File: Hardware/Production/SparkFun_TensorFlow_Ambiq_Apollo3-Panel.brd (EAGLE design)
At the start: 175.6 x 134.7 mm, 906 parts, among them J12 CORTEX_DEBUG, J14 CAMERA-OV7670, J18 CORTEX_DEBUG, J20 CAMERA-OV7670, J24 CORTEX_DEBUG, J26 CAMERA-OV7670, J30 CORTEX_DEBUG, J32 CAMERA-OV7670, J36 CORTEX_DEBUG, J38 CAMERA-OV7670, J42 CORTEX_DEBUG, J44 CAMERA-OV7670, J48 CORTEX_DEBUG, J5 CORTEX_DEBUG, J50 CAMERA-OV7670, J54 CORTEX_DEBUG, J6 CAMERA-OV7670, J8 CAMERA-OV7670, U1 LIS2DH12, U10 LIS2DH12, U11 1.8V, U12 ARTEMIS_MODULESMD, U13 LIS2DH12, U14 1.8V, U15 ARTEMIS_MODULESMD, U16 LIS2DH12, U17 1.8V, U18 ARTEMIS_MODULESMD, U19 LIS2DH12, U2 LIS2DH12, U20 1.8V, U21 ARTEMIS_MODULESMD, U22 LIS2DH12, U23 1.8V, U24 ARTEMIS_MODULESMD, U25 LIS2DH12, U26 1.8V, U27 ARTEMIS_MODULESMD, U3 1.8V, U4 1.8V, U5 ARTEMIS_MODULESMD, U6 ARTEMIS_MODULESMD, U7 LIS2DH12, U8 1.8V, U9 ARTEMIS_MODULESMD, Y1 32.768kHz, Y2 32.768kHz, Y3 32.768kHz, Y4 32.768kHz, Y5 32.768kHz, Y6 32.768kHz, Y7 32.768kHz, Y8 32.768kHz, Y9 32.768kHz

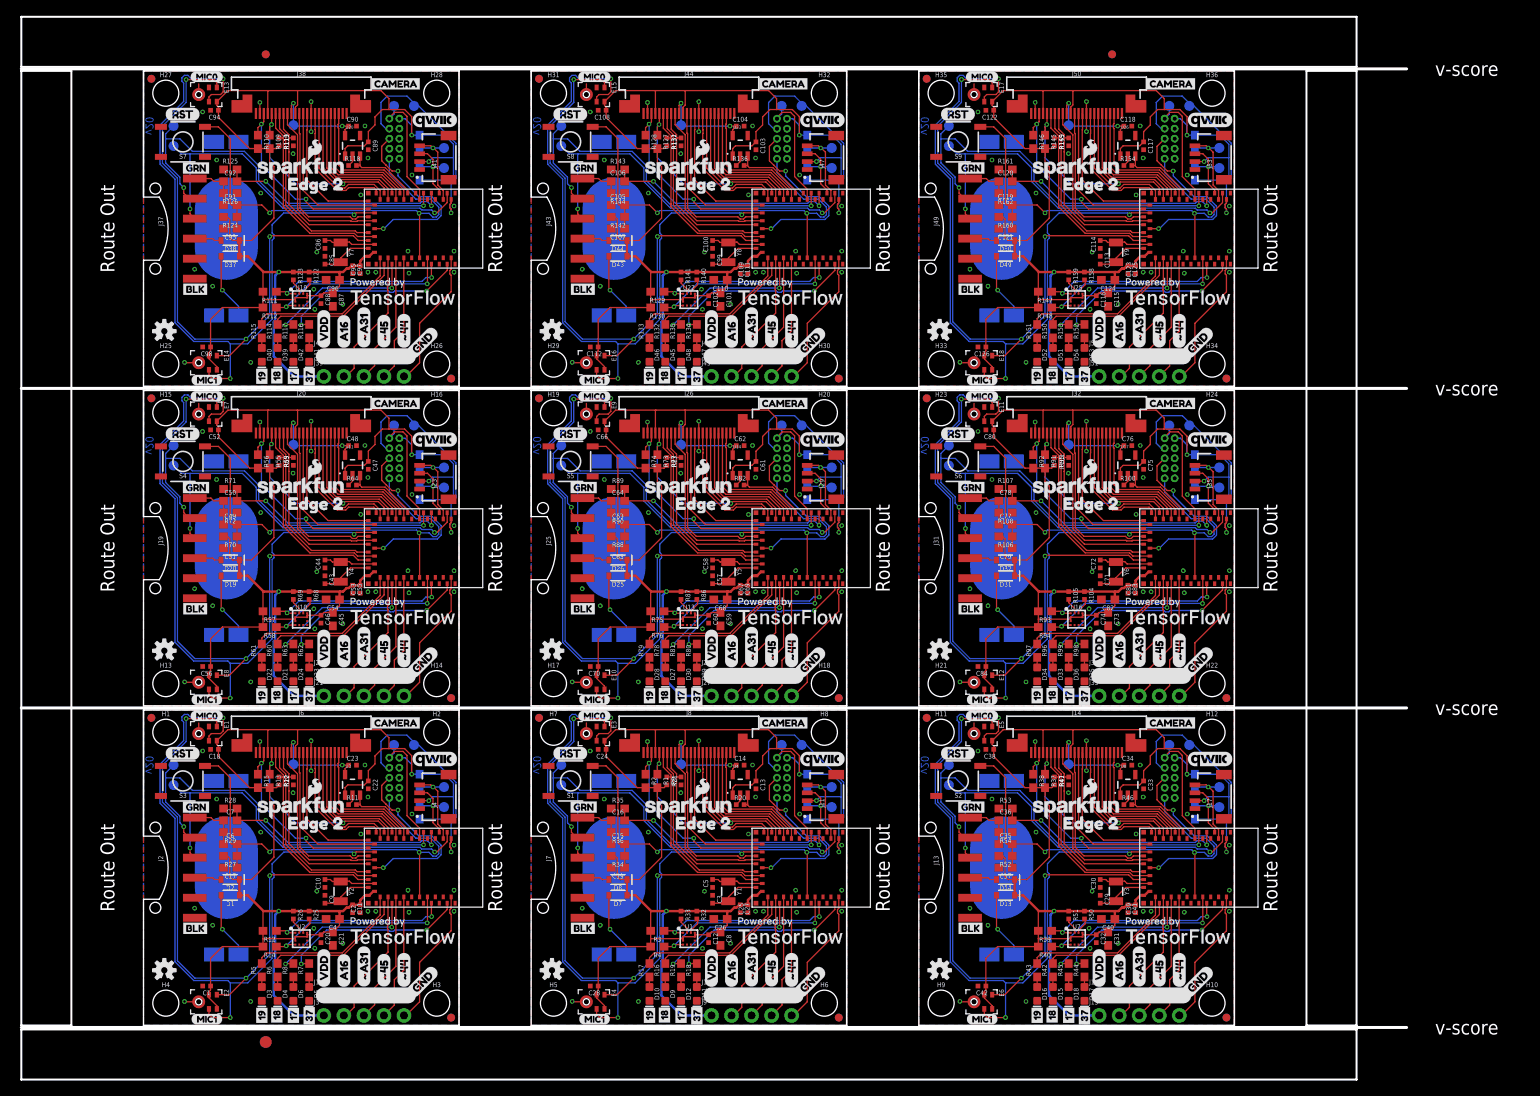
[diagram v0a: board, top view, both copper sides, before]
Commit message: Adding panel files for v2.1
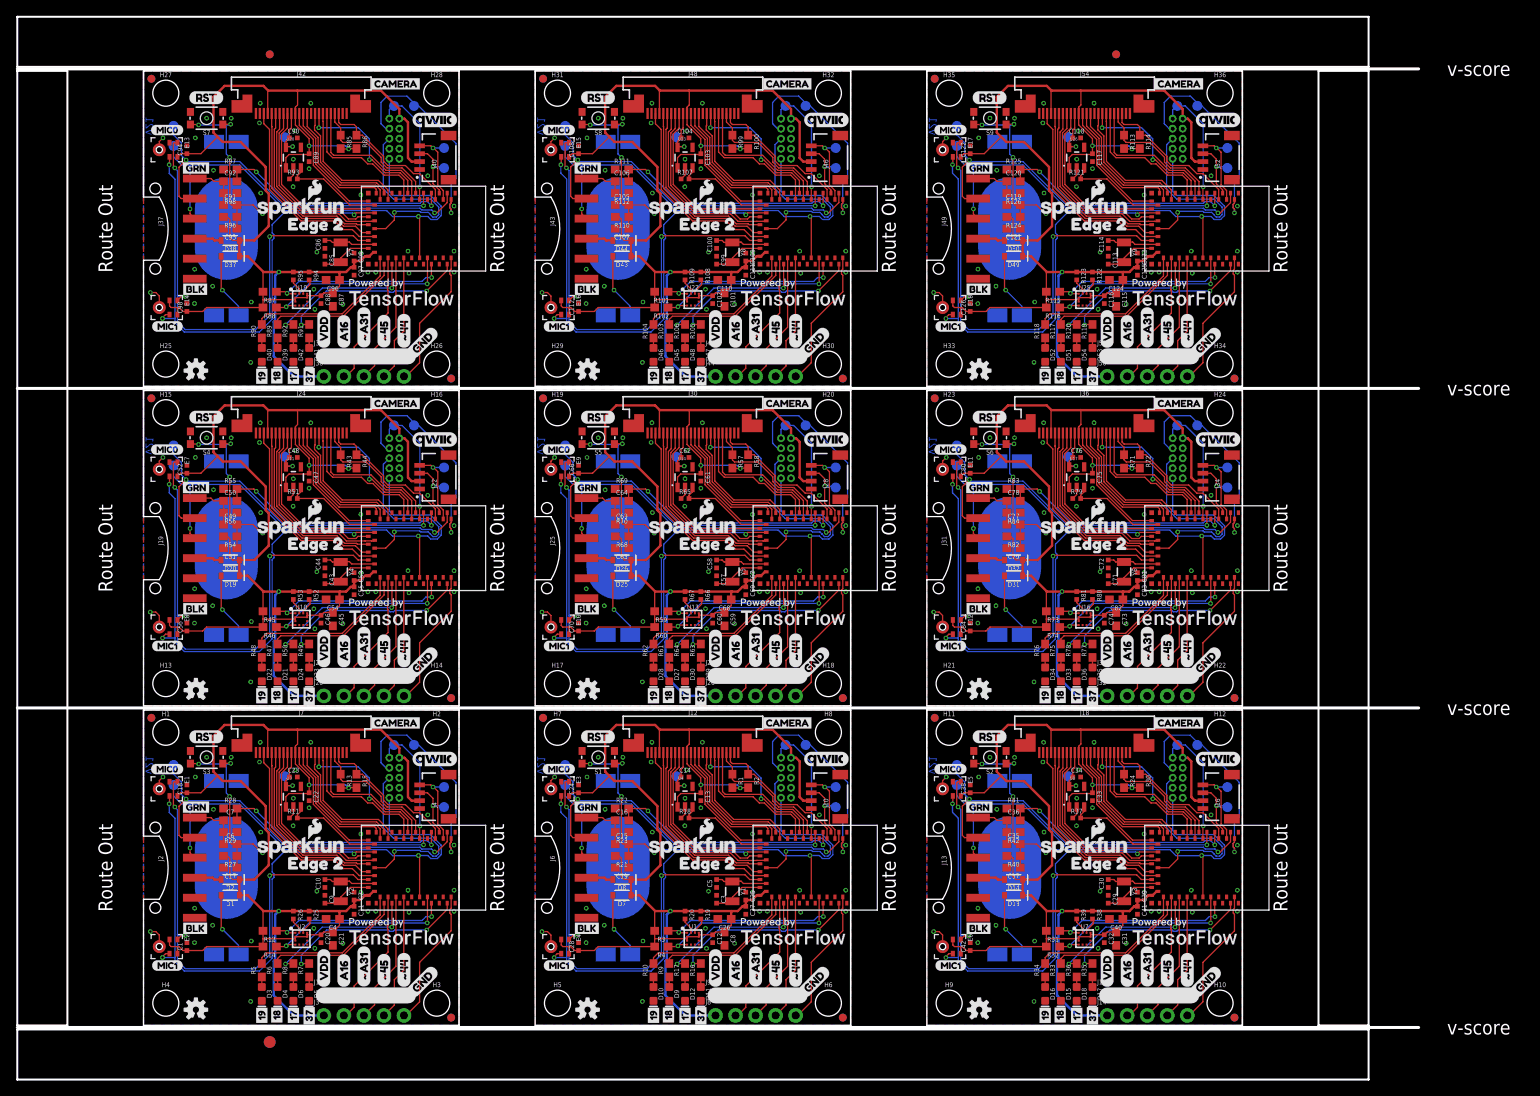
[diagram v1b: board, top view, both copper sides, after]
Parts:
- removed R127, R128, R129, R130, R138, R139, R145, R146, R147, R148, R156, R157: 4.7k, SparkFun-Resistors:0603
- removed R131, R136, R137, R140, R141, R149, R154, R155, R158, R159: 10k, SparkFun-Resistors:0402-TIGHT
- removed R132, R133, R134, R135, R150, R151, R152, R153: 1k, SparkFun-Resistors:0603
- removed R142, R144, R160, R162: 100k, SparkFun-Resistors:0603
- removed R143, R161: 10k, SparkFun-Resistors:0603
- J10, J16, J22, J28, J34, J40, J46, J52: device SparkFun-Connectors:1X05_NO_SILK -> SparkFun-Connectors:JST04_1MM_RA
- J11, J17, J23, J29, J35, J41, J47, J53: value (none) -> CORTEX_DEBUG; device SparkFun-Connectors:JST04_1MM_RA -> SparkFun-Connectors:2X5-PTH-1.27MM
- J12, J18, J24, J30, J36, J42, J48, J54: value CORTEX_DEBUG -> CAMERA-HIMAX; device SparkFun-Connectors:2X5-PTH-1.27MM -> SparkFun-Connectors:FPC-24-AMPHENOL-SFV24R-1STE1HLF
- J14, J20, J26, J32, J38, J44, J50, J8: value CAMERA-OV7670 -> (none); device SparkFun-Connectors:FPC-24-AMPHENOL-SFV24R-1STE1HLF -> SparkFun-Connectors:1X05_NO_SILK
- J6: value CAMERA-OV7670 -> (none); device SparkFun-Connectors:FPC-24-AMPHENOL-SFV24R-1STE1HLF -> SparkFun-Connectors:1X06-SMD_RA_MALE
- J7: value (none) -> CAMERA-HIMAX; device SparkFun-Connectors:1X06-SMD_RA_MALE -> SparkFun-Connectors:FPC-24-AMPHENOL-SFV24R-1STE1HLF
- R10, R104, R105, R118, R119, R33, R47, R50, R64, R77, R9: value 10k -> 1k; device SparkFun-Resistors:0402-TIGHT -> SparkFun-Resistors:0603
- R100, R101, R113, R32, R46, R59, R86, R87: value 10k -> 4.7k; device SparkFun-Resistors:0402-TIGHT -> SparkFun-Resistors:0603
- R103, R120, R48, R49, R75, R76, R91, R92: value 4.7k -> 1k
- R106, R34, R36, R90: value 100k -> 1k
- R107, R53: device SparkFun-Resistors:0603 -> SparkFun-Resistors:0402-TIGHT
- R108, R52: value 100k -> 10k; device SparkFun-Resistors:0603 -> SparkFun-Resistors:0402-TIGHT
- R109, R121, R37, R38, R39, R66, R67, R93, R94: value 4.7k -> 10k; device SparkFun-Resistors:0603 -> SparkFun-Resistors:0402-TIGHT
- R110, R112, R23, R40, R56, R84: value 4.7k -> 100k
- R111, R55: value 4.7k -> 10k
- R114, R115, R116, R43, R44, R45, R60, R99: value 1k -> 4.7k
- R18, R19, R79, R80, R81: value 1k -> 10k; device SparkFun-Resistors:0603 -> SparkFun-Resistors:0402-TIGHT
- R21, R68, R82: value 10k -> 100k; device SparkFun-Resistors:0402-TIGHT -> SparkFun-Resistors:0603
- R22, R41, R69, R83: device SparkFun-Resistors:0402-TIGHT -> SparkFun-Resistors:0603
- R35, R89: value 10k -> 1k
- R42, R96, R98: value 1k -> 100k
- R71: value 10k -> 4.7k
- R72, R88: value 100k -> 4.7k
- R97: value 1k -> 10k
- S1, S2, S3, S4, S5, S6, S7, S8, S9: device SparkFun-Switches:TACTILE_SWITCH_SMD_5.2MM -> SparkFun-Switches:TACTILE_SWITCH_SMD_4.6X2.8MM
- U12, U15, U18, U21, U24, U27, U5, U6, U9: device Testing:ARTEMIS_FP -> SparkFun-IC-Microcontroller:ARTEMIS_FP
- moved R98 122.8 mm to (11.0, 105.5), turned to 180 degrees
- moved R48 120.1 mm to (15.0, 47.5), flipped to the top, turned to 90 degrees
- moved R97 119.1 mm to (11.0, 108.5), turned to 0 degrees
- moved R96 117.9 mm to (11.0, 102.5), turned to 180 degrees
- moved R72 115.5 mm to (126.3, 71.5), turned to 270 degrees
- moved R49 113.5 mm to (21.0, 47.5), flipped to the top
- moved R71 113.4 mm to (124.3, 71.5), turned to 270 degrees
- moved R44 112.6 mm to (27.0, 71.5), turned to 270 degrees
- moved R114 111.9 mm to (126.3, 112.0), turned to 270 degrees
- moved R51 111.6 mm to (19.0, 66.8), turned to 0 degrees
- moved R46 111.1 mm to (16.0, 50.5), turned to 180 degrees
- moved R45 111.0 mm to (16.0, 52.5), turned to 180 degrees
- moved R93 109.9 mm to (19.0, 107.3), turned to 0 degrees
- moved R43 109.3 mm to (25.0, 71.5), turned to 270 degrees
- moved R113 107.1 mm to (124.3, 112.0)
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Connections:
- removed net CAMERA_HREF: J6.9, U5.~AD13
- removed net CAMERA_HREF1: J8.9, U6.~AD13
- removed net CAMERA_HREF2: J14.9, U9.~AD13
- removed net CAMERA_HREF3: J20.9, U12.~AD13
- removed net CAMERA_HREF4: J26.9, U15.~AD13
- removed net CAMERA_HREF5: J32.9, U18.~AD13
- removed net CAMERA_HREF6: J38.9, U21.~AD13
- removed net CAMERA_HREF7: J44.9, U24.~AD13
- removed net CAMERA_HREF8: J50.9, U27.~AD13
- removed net CAMERA_PWDN: J6.8, R22.2, U5.D15
- removed net CAMERA_PWDN1: J8.8, R21.2, U6.D15
- removed net CAMERA_PWDN2: J14.8, R47.2, U9.D15
- removed net CAMERA_PWDN3: J20.8, R65.2, U12.D15
- removed net CAMERA_PWDN4: J26.8, R83.2, U15.D15
- removed net CAMERA_PWDN5: J32.8, R101.2, U18.D15
- removed net CAMERA_PWDN6: J38.8, R119.2, U21.D15
- removed net CAMERA_PWDN7: J44.8, R137.2, U24.D15
- removed net CAMERA_PWDN8: J50.8, R155.2, U27.D15
- removed net CAMERA_RESET: J6.6, R10.1, U5.~AD11
- removed net CAMERA_RESET1: J8.6, R9.1, U6.~AD11
- removed net CAMERA_RESET2: J14.6, R41.1, U9.~AD11
- removed net CAMERA_RESET3: J20.6, R59.1, U12.~AD11
- removed net CAMERA_RESET4: J26.6, R77.1, U15.~AD11
- removed net CAMERA_RESET5: J32.6, R95.1, U18.~AD11
- removed net CAMERA_RESET6: J38.6, R113.1, U21.~AD11
- removed net CAMERA_RESET7: J44.6, R131.1, U24.~AD11
- removed net CAMERA_RESET8: J50.6, R149.1, U27.~AD11
- removed net CAMERA_XCLK: J6.13, U5.~AD32
- removed net CAMERA_XCLK1: J8.13, U6.~AD32
- removed net CAMERA_XCLK2: J14.13, U9.~AD32
- removed net CAMERA_XCLK3: J20.13, U12.~AD32
- removed net CAMERA_XCLK4: J26.13, U15.~AD32
- removed net CAMERA_XCLK5: J32.13, U18.~AD32
- removed net CAMERA_XCLK6: J38.13, U21.~AD32
- removed net CAMERA_XCLK7: J44.13, U24.~AD32
- removed net CAMERA_XCLK8: J50.13, U27.~AD32
- removed net CAMERA_Y0: J6.19, U5.~D22
- removed net CAMERA_Y1: J6.21, U5.~D4
- removed net CAMERA_Y10: J8.22, U6.~AD35
- removed net CAMERA_Y11: J8.18, U6.~D23
- removed net CAMERA_Y12: J8.19, U6.~D22
- removed net CAMERA_Y13: J8.12, U6.~D26
- removed net CAMERA_Y14: J8.14, U6.~D6
- removed net CAMERA_Y15: J8.16, U6.~D28
- removed net CAMERA_Y16: J14.20, U9.~D24
- removed net CAMERA_Y17: J14.21, U9.~D4
- removed net CAMERA_Y18: J14.22, U9.~AD35
- removed net CAMERA_Y19: J14.18, U9.~D23
- removed net CAMERA_Y2: J6.22, U5.~AD35
- removed net CAMERA_Y20: J14.19, U9.~D22
- removed net CAMERA_Y21: J14.12, U9.~D26
- removed net CAMERA_Y22: J14.14, U9.~D6
- removed net CAMERA_Y23: J14.16, U9.~D28
- removed net CAMERA_Y24: J20.20, U12.~D24
- removed net CAMERA_Y25: J20.21, U12.~D4
- removed net CAMERA_Y26: J20.22, U12.~AD35
- removed net CAMERA_Y27: J20.18, U12.~D23
- removed net CAMERA_Y28: J20.19, U12.~D22
- removed net CAMERA_Y29: J20.12, U12.~D26
- removed net CAMERA_Y3: J6.20, U5.~D24
- removed net CAMERA_Y30: J20.14, U12.~D6
- removed net CAMERA_Y31: J20.16, U12.~D28
- removed net CAMERA_Y32: J26.20, U15.~D24
- removed net CAMERA_Y33: J26.21, U15.~D4
- removed net CAMERA_Y34: J26.22, U15.~AD35
- removed net CAMERA_Y35: J26.18, U15.~D23
- removed net CAMERA_Y36: J26.19, U15.~D22
- removed net CAMERA_Y37: J26.12, U15.~D26
- removed net CAMERA_Y38: J26.14, U15.~D6
- removed net CAMERA_Y39: J26.16, U15.~D28
- removed net CAMERA_Y4: J6.18, U5.~D23
- removed net CAMERA_Y40: J32.20, U18.~D24
- removed net CAMERA_Y41: J32.21, U18.~D4
- removed net CAMERA_Y42: J32.22, U18.~AD35
- removed net CAMERA_Y43: J32.18, U18.~D23
- removed net CAMERA_Y44: J32.19, U18.~D22
- removed net CAMERA_Y45: J32.12, U18.~D26
- removed net CAMERA_Y46: J32.14, U18.~D6
- removed net CAMERA_Y47: J32.16, U18.~D28
- removed net CAMERA_Y48: J38.20, U21.~D24
- removed net CAMERA_Y49: J38.21, U21.~D4
- removed net CAMERA_Y5: J6.16, U5.~D28
- removed net CAMERA_Y50: J38.22, U21.~AD35
- removed net CAMERA_Y51: J38.18, U21.~D23
- removed net CAMERA_Y52: J38.19, U21.~D22
- removed net CAMERA_Y53: J38.12, U21.~D26
- removed net CAMERA_Y54: J38.14, U21.~D6
- removed net CAMERA_Y55: J38.16, U21.~D28
- removed net CAMERA_Y56: J44.20, U24.~D24
- removed net CAMERA_Y57: J44.21, U24.~D4
- removed net CAMERA_Y58: J44.22, U24.~AD35
- removed net CAMERA_Y59: J44.18, U24.~D23
- removed net CAMERA_Y6: J6.14, U5.~D6
- removed net CAMERA_Y60: J44.19, U24.~D22
- removed net CAMERA_Y61: J44.12, U24.~D26
- removed net CAMERA_Y62: J44.14, U24.~D6
- removed net CAMERA_Y63: J44.16, U24.~D28
- removed net CAMERA_Y64: J50.20, U27.~D24
- removed net CAMERA_Y65: J50.21, U27.~D4
- removed net CAMERA_Y66: J50.22, U27.~AD35
- removed net CAMERA_Y67: J50.18, U27.~D23
- removed net CAMERA_Y68: J50.19, U27.~D22
- removed net CAMERA_Y69: J50.12, U27.~D26
- removed net CAMERA_Y7: J6.12, U5.~D26
- removed net CAMERA_Y70: J50.14, U27.~D6
- removed net CAMERA_Y71: J50.16, U27.~D28
- removed net CAMERA_Y8: J8.20, U6.~D24
- removed net CAMERA_Y9: J8.21, U6.~D4
- new net CAMERA_D0: J7.14, U5.D14
- new net CAMERA_D1: J7.3, U5.~AD11
- new net CAMERA_D10: J12.9, U6.~D25
- new net CAMERA_D11: J12.12, U6.~D6
- new net CAMERA_D12: J12.14, U6.D14
- new net CAMERA_D13: J12.13, U6.~D28
- new net CAMERA_D14: J12.19, U6.~AD35
- new net CAMERA_D15: J12.20, U6.~D5
- new net CAMERA_D16: J18.5, U9.AD34
- new net CAMERA_D17: J18.3, U9.~AD11
- new net CAMERA_D18: J18.9, U9.~D25
- new net CAMERA_D19: J18.12, U9.~D6
- new net CAMERA_D2: J7.9, U5.~D25
- new net CAMERA_D20: J18.14, U9.D14
- new net CAMERA_D21: J18.13, U9.~D28
- new net CAMERA_D22: J18.19, U9.~AD35
- new net CAMERA_D23: J18.20, U9.~D5
- new net CAMERA_D24: J24.5, U12.AD34
- new net CAMERA_D25: J24.3, U12.~AD11
- new net CAMERA_D26: J24.9, U12.~D25
- new net CAMERA_D27: J24.12, U12.~D6
- new net CAMERA_D28: J24.14, U12.D14
- new net CAMERA_D29: J24.13, U12.~D28
- new net CAMERA_D3: J7.5, U5.AD34
- new net CAMERA_D30: J24.19, U12.~AD35
- new net CAMERA_D31: J24.20, U12.~D5
- new net CAMERA_D32: J30.5, U15.AD34
- new net CAMERA_D33: J30.3, U15.~AD11
- new net CAMERA_D34: J30.9, U15.~D25
- new net CAMERA_D35: J30.12, U15.~D6
- new net CAMERA_D36: J30.14, U15.D14
- new net CAMERA_D37: J30.13, U15.~D28
- new net CAMERA_D38: J30.19, U15.~AD35
- new net CAMERA_D39: J30.20, U15.~D5
- new net CAMERA_D4: J7.12, U5.~D6
- new net CAMERA_D40: J36.5, U18.AD34
- new net CAMERA_D41: J36.3, U18.~AD11
- new net CAMERA_D42: J36.9, U18.~D25
- new net CAMERA_D43: J36.12, U18.~D6
- new net CAMERA_D44: J36.14, U18.D14
- new net CAMERA_D45: J36.13, U18.~D28
- new net CAMERA_D46: J36.19, U18.~AD35
- new net CAMERA_D47: J36.20, U18.~D5
- new net CAMERA_D48: J42.5, U21.AD34
- new net CAMERA_D49: J42.3, U21.~AD11
- new net CAMERA_D5: J7.20, U5.~D5
- new net CAMERA_D50: J42.9, U21.~D25
- new net CAMERA_D51: J42.12, U21.~D6
- new net CAMERA_D52: J42.14, U21.D14
- new net CAMERA_D53: J42.13, U21.~D28
- new net CAMERA_D54: J42.19, U21.~AD35
- new net CAMERA_D55: J42.20, U21.~D5
- new net CAMERA_D56: J48.5, U24.AD34
- new net CAMERA_D57: J48.3, U24.~AD11
- new net CAMERA_D58: J48.9, U24.~D25
- new net CAMERA_D59: J48.12, U24.~D6
- new net CAMERA_D6: J7.19, U5.~AD35
- new net CAMERA_D60: J48.14, U24.D14
- new net CAMERA_D61: J48.13, U24.~D28
- new net CAMERA_D62: J48.19, U24.~AD35
- new net CAMERA_D63: J48.20, U24.~D5
- new net CAMERA_D64: J54.5, U27.AD34
- new net CAMERA_D65: J54.3, U27.~AD11
- new net CAMERA_D66: J54.9, U27.~D25
- new net CAMERA_D67: J54.12, U27.~D6
- new net CAMERA_D68: J54.14, U27.D14
- new net CAMERA_D69: J54.13, U27.~D28
- new net CAMERA_D7: J7.13, U5.~D28
- new net CAMERA_D70: J54.19, U27.~AD35
- new net CAMERA_D71: J54.20, U27.~D5
- new net CAMERA_D8: J12.5, U6.AD34
- new net CAMERA_D9: J12.3, U6.~AD11
- new net CAMERA_HSYNC: J7.16, U5.~D27
- new net CAMERA_HSYNC1: J12.16, U6.~D27
- new net CAMERA_HSYNC2: J18.16, U9.~D27
- new net CAMERA_HSYNC3: J24.16, U12.~D27
- new net CAMERA_HSYNC4: J30.16, U15.~D27
- new net CAMERA_HSYNC5: J36.16, U18.~D27
- new net CAMERA_HSYNC6: J42.16, U21.~D27
- new net CAMERA_HSYNC7: J48.16, U24.~D27
- new net CAMERA_HSYNC8: J54.16, U27.~D27
- new net CAMERA_INT: J7.18, U5.~D23
- new net CAMERA_INT1: J12.18, U6.~D23
- new net CAMERA_INT2: J18.18, U9.~D23
- new net CAMERA_INT3: J24.18, U12.~D23
- new net CAMERA_INT4: J30.18, U15.~D23
- new net CAMERA_INT5: J36.18, U18.~D23
- new net CAMERA_INT6: J42.18, U21.~D23
- new net CAMERA_INT7: J48.18, U24.~D23
- new net CAMERA_INT8: J54.18, U27.~D23
- new net CAMERA_MCLK: J7.8, U5.~D26
- new net CAMERA_MCLK1: J12.8, U6.~D26
- new net CAMERA_MCLK2: J18.8, U9.~D26
- new net CAMERA_MCLK3: J24.8, U12.~D26
- new net CAMERA_MCLK4: J30.8, U15.~D26
- new net CAMERA_MCLK5: J36.8, U18.~D26
- new net CAMERA_MCLK6: J42.8, U21.~D26
- new net CAMERA_MCLK7: J48.8, U24.~D26
- new net CAMERA_MCLK8: J54.8, U27.~D26
- new net CAMERA_TRIG: J7.7, U5.~AD13
- new net CAMERA_TRIG1: J12.7, U6.~AD13
- new net CAMERA_TRIG2: J18.7, U9.~AD13
- new net CAMERA_TRIG3: J24.7, U12.~AD13
- new net CAMERA_TRIG4: J30.7, U15.~AD13
- new net CAMERA_TRIG5: J36.7, U18.~AD13
- new net CAMERA_TRIG6: J42.7, U21.~AD13
- new net CAMERA_TRIG7: J48.7, U24.~AD13
- new net CAMERA_TRIG8: J54.7, U27.~AD13
- net !DTR1: now also J6.1, R23.2; no longer J7.1, R36.2
- net !DTR2: now also R42.2; no longer R54.2
- net !DTR3: now also R56.2; no longer R72.2
- net !DTR4: now also R70.2; no longer R90.2
- net !DTR5: now also R84.2; no longer R108.2
- net !DTR6: now also R98.2; no longer R126.2
- net !DTR7: now also R112.2; no longer R144.2
- net !DTR8: now also R126.2; no longer R162.2
- net 1.8V: now also J7.10; no longer J6.10
- net 1.8V1: now also J12.10; no longer J8.10
- net 1.8V2: now also J18.10; no longer J14.10
- net 1.8V3: now also J24.10; no longer J20.10
- net 1.8V4: now also J30.10; no longer J26.10
- net 1.8V5: now also J36.10; no longer J32.10
- net 1.8V6: now also J42.10; no longer J38.10
- net 1.8V7: now also J48.10; no longer J44.10
- net 1.8V8: now also J54.10; no longer J50.10
- net A1: now also J8.2; no longer J9.2
- net A2: now also J14.2; no longer J15.2
- net A3: now also J20.2; no longer J21.2
- net A4: now also J26.2; no longer J27.2
- net A5: now also J32.2; no longer J33.2
- net A6: now also J38.2; no longer J39.2
- net A7: now also J44.2; no longer J45.2
- net A8: now also J50.2; no longer J51.2
- net ACCEL_I2C_SCL2: now also R31.1; no longer R39.1
- net ACCEL_I2C_SCL3: now also R45.1; no longer R57.1
- net ACCEL_I2C_SCL4: now also R59.1; no longer R75.1
- net ACCEL_I2C_SCL5: now also R73.1; no longer R93.1
- net ACCEL_I2C_SCL6: now also R87.1; no longer R111.1
- net ACCEL_I2C_SCL7: now also R101.1; no longer R129.1
- net ACCEL_I2C_SCL8: now also R115.1; no longer R147.1
- net ACCEL_I2C_SDA2: now also R32.1; no longer R40.1
- net ACCEL_I2C_SDA3: now also R46.1; no longer R58.1
- net ACCEL_I2C_SDA4: now also R60.1; no longer R76.1
- net ACCEL_I2C_SDA5: now also R74.1; no longer R94.1
- net ACCEL_I2C_SDA6: now also R88.1; no longer R112.1
- net ACCEL_I2C_SDA7: now also R102.1; no longer R130.1
- net ACCEL_I2C_SDA8: now also R116.1; no longer R148.1
- net ACCEL_INT10: now also R66.2; no longer R86.2
- net ACCEL_INT11: now also R81.2; no longer R105.2
- net ACCEL_INT12: now also R80.2; no longer R104.2
- net ACCEL_INT13: now also R95.2; no longer R123.2
- net ACCEL_INT14: now also R94.2; no longer R122.2
- net ACCEL_INT15: now also R109.2; no longer R141.2
- net ACCEL_INT16: now also R108.2; no longer R140.2
- net ACCEL_INT17: now also R123.2; no longer R159.2
- net ACCEL_INT18: now also R122.2; no longer R158.2
- net ACCEL_INT3: now also R20.2; no longer R33.2
- net ACCEL_INT4: now also R19.2; no longer R32.2
- net ACCEL_INT5: now also R39.2; no longer R51.2
- net ACCEL_INT6: now also R38.2; no longer R50.2
- net ACCEL_INT7: now also R53.2; no longer R69.2
- net ACCEL_INT8: now also R52.2; no longer R68.2
- net ACCEL_INT9: now also R67.2; no longer R87.2
- net AMBIQ_!RST: now also S3.4
- net AMBIQ_!RST1: now also J11.10, R21.1, S1.4; no longer J12.10, R34.1
- net AMBIQ_!RST2: now also J17.10, R40.1, S2.4; no longer J18.10, R52.1
- net AMBIQ_!RST3: now also J23.10, R54.1, S4.4; no longer J24.10, R70.1
- net AMBIQ_!RST4: now also J29.10, R68.1, S5.4; no longer J30.10, R88.1
- net AMBIQ_!RST5: now also J35.10, R82.1, S6.4; no longer J36.10, R106.1
- net AMBIQ_!RST6: now also J41.10, R96.1, S7.4; no longer J42.10, R124.1
- net AMBIQ_!RST7: now also J47.10, R110.1, S8.4; no longer J48.10, R142.1
- net AMBIQ_!RST8: now also J53.10, R124.1, S9.4; no longer J54.10, R160.1
- net BOOT1: now also R22.2; no longer R35.2
- net BOOT2: now also R41.2; no longer R53.2
- net BOOT3: now also R55.2; no longer R71.2
- net BOOT4: now also R69.2; no longer R89.2
- net BOOT5: now also R83.2; no longer R107.2
- net BOOT6: now also R97.2; no longer R125.2
- net BOOT7: now also R111.2; no longer R143.2
- net BOOT8: now also R125.2; no longer R161.2
- net CAMERA_DVDD_EN: now also U5.~AD32; no longer U5.D7
- net CAMERA_DVDD_EN1: now also R18.2, U6.~AD32; no longer R20.2, U6.D7
- net CAMERA_DVDD_EN2: now also R37.2, U9.~AD32; no longer R46.2, U9.D7
- net CAMERA_DVDD_EN3: now also R51.2, U12.~AD32; no longer R64.2, U12.D7
- net CAMERA_DVDD_EN4: now also R65.2, U15.~AD32; no longer R82.2, U15.D7
- net CAMERA_DVDD_EN5: now also R79.2, U18.~AD32; no longer R100.2, U18.D7
- net CAMERA_DVDD_EN6: now also R93.2, U21.~AD32; no longer R118.2, U21.D7
- net CAMERA_DVDD_EN7: now also R107.2, U24.~AD32; no longer R136.2, U24.D7
- net CAMERA_DVDD_EN8: now also R121.2, U27.~AD32; no longer R154.2, U27.D7
- net CAMERA_I2C_SCL: now also J7.21, U5.D8; no longer J6.5, U5.~D27
- net CAMERA_I2C_SCL1: now also J12.21, U6.D8; no longer J8.5, U6.~D27
- net CAMERA_I2C_SCL2: now also J18.21, R24.1, U9.D8; no longer J14.5, R37.1, U9.~D27
- net CAMERA_I2C_SCL3: now also J24.21, R43.1, U12.D8; no longer J20.5, R55.1, U12.~D27
- net CAMERA_I2C_SCL4: now also J30.21, R57.1, U15.D8; no longer J26.5, R73.1, U15.~D27
- net CAMERA_I2C_SCL5: now also J36.21, R71.1, U18.D8; no longer J32.5, R91.1, U18.~D27
- net CAMERA_I2C_SCL6: now also J42.21, R85.1, U21.D8; no longer J38.5, R109.1, U21.~D27
- net CAMERA_I2C_SCL7: now also J48.21, R99.1, U24.D8; no longer J44.5, R127.1, U24.~D27
- net CAMERA_I2C_SCL8: now also J54.21, R113.1, U27.D8; no longer J50.5, R145.1, U27.~D27
- net CAMERA_I2C_SDA: now also J7.22, U5.D9; no longer J6.3, U5.~D25
- net CAMERA_I2C_SDA1: now also J12.22, U6.D9; no longer J8.3, U6.~D25
- net CAMERA_I2C_SDA2: now also J18.22, R30.1, U9.D9; no longer J14.3, R38.1, U9.~D25
- net CAMERA_I2C_SDA3: now also J24.22, R44.1, U12.D9; no longer J20.3, R56.1, U12.~D25
- net CAMERA_I2C_SDA4: now also J30.22, R58.1, U15.D9; no longer J26.3, R74.1, U15.~D25
- net CAMERA_I2C_SDA5: now also J36.22, R72.1, U18.D9; no longer J32.3, R92.1, U18.~D25
- net CAMERA_I2C_SDA6: now also J42.22, R86.1, U21.D9; no longer J38.3, R110.1, U21.~D25
- net CAMERA_I2C_SDA7: now also J48.22, R100.1, U24.D9; no longer J44.3, R128.1, U24.~D25
- net CAMERA_I2C_SDA8: now also J54.22, R114.1, U27.D9; no longer J50.3, R146.1, U27.~D25
- net CAMERA_PCLK: now also J7.17, U5.D7; no longer J6.17, U5.D14
- net CAMERA_PCLK1: now also J12.17, U6.D7; no longer J8.17, U6.D14
- net CAMERA_PCLK2: now also J18.17, U9.D7; no longer J14.17, U9.D14
- net CAMERA_PCLK3: now also J24.17, U12.D7; no longer J20.17, U12.D14
- net CAMERA_PCLK4: now also J30.17, U15.D7; no longer J26.17, U15.D14
- net CAMERA_PCLK5: now also J36.17, U18.D7; no longer J32.17, U18.D14
- net CAMERA_PCLK6: now also J42.17, U21.D7; no longer J38.17, U21.D14
- net CAMERA_PCLK7: now also J48.17, U24.D7; no longer J44.17, U24.D14
- net CAMERA_PCLK8: now also J54.17, U27.D7; no longer J50.17, U27.D14
- net CAMERA_VSYNC: now also J7.6, U5.D15; no longer J6.7, U5.AD34
- net CAMERA_VSYNC1: now also J12.6, U6.D15; no longer J8.7, U6.AD34
- net CAMERA_VSYNC2: now also J18.6, U9.D15; no longer J14.7, U9.AD34
- net CAMERA_VSYNC3: now also J24.6, U12.D15; no longer J20.7, U12.AD34
- net CAMERA_VSYNC4: now also J30.6, U15.D15; no longer J26.7, U15.AD34
- net CAMERA_VSYNC5: now also J36.6, U18.D15; no longer J32.7, U18.AD34
- net CAMERA_VSYNC6: now also J42.6, U21.D15; no longer J38.7, U21.AD34
- net CAMERA_VSYNC7: now also J48.6, U24.D15; no longer J44.7, U24.AD34
- net CAMERA_VSYNC8: now also J54.6, U27.D15; no longer J50.7, U27.AD34
- net FTDI_VCC1: now also J6.4; no longer J7.4
- net GND: now also J7.15, J7.2, S3.2; no longer J6.15, J6.2, R22.1
- net GND1: now also J11.3, J11.5, J11.9, J12.15, J12.2, J6.6, J9.1, J9.2, J9.3, J9.4, J9.5, R18.1, R22.1, R23.1, S1.2; no longer J10.2, J10.3, J10.4, J10.5, J11.1, J12.3, J12.5, J12.9, J7.6, J8.15, J8.2, R20.1, R21.1, R35.1, R36.1
- net GND2: now also J15.1, J15.2, J15.3, J15.4, J15.5, J17.3, J17.5, J17.9, J18.15, J18.2, R37.1, R41.1, R42.1, S2.2; no longer J14.15, J14.2, J16.2, J16.3, J16.4, J16.5, J17.1, J18.3, J18.5, J18.9, R46.1, R47.1, R53.1, R54.1
- net GND3: now also J21.1, J21.2, J21.3, J21.4, J21.5, J23.3, J23.5, J23.9, J24.15, J24.2, R51.1, R55.1, R56.1, S4.2; no longer J20.15, J20.2, J22.2, J22.3, J22.4, J22.5, J23.1, J24.3, J24.5, J24.9, R64.1, R65.1, R71.1, R72.1
- net GND4: now also J27.1, J27.2, J27.3, J27.4, J27.5, J29.3, J29.5, J29.9, J30.15, J30.2, R65.1, R69.1, R70.1, S5.2; no longer J26.15, J26.2, J28.2, J28.3, J28.4, J28.5, J29.1, J30.3, J30.5, J30.9, R82.1, R83.1, R89.1, R90.1
- net GND5: now also J33.1, J33.2, J33.3, J33.4, J33.5, J35.3, J35.5, J35.9, J36.15, J36.2, R79.1, R83.1, R84.1, S6.2; no longer J32.15, J32.2, J34.2, J34.3, J34.4, J34.5, J35.1, J36.3, J36.5, J36.9, R100.1, R101.1, R107.1, R108.1
- net GND6: now also J39.1, J39.2, J39.3, J39.4, J39.5, J41.3, J41.5, J41.9, J42.15, J42.2, R93.1, R97.1, R98.1, S7.2; no longer J38.15, J38.2, J40.2, J40.3, J40.4, J40.5, J41.1, J42.3, J42.5, J42.9, R118.1, R119.1, R125.1, R126.1
- net GND7: now also J45.1, J45.2, J45.3, J45.4, J45.5, J47.3, J47.5, J47.9, J48.15, J48.2, R107.1, R111.1, R112.1, S8.2; no longer J44.15, J44.2, J46.2, J46.3, J46.4, J46.5, J47.1, J48.3, J48.5, J48.9, R136.1, R137.1, R143.1, R144.1
- net GND8: now also J51.1, J51.2, J51.3, J51.4, J51.5, J53.3, J53.5, J53.9, J54.15, J54.2, R121.1, R125.1, R126.1, S9.2; no longer J50.15, J50.2, J52.2, J52.3, J52.4, J52.5, J53.1, J54.3, J54.5, J54.9, R154.1, R155.1, R161.1, R162.1
- net LED_BLUE1: now also R9.2; no longer R16.2
- net LED_BLUE2: now also R33.2; no longer R42.2
- net LED_BLUE3: now also R47.2; no longer R60.2
- net LED_BLUE4: now also R61.2; no longer R78.2
- net LED_BLUE5: now also R75.2; no longer R96.2
- net LED_BLUE6: now also R89.2; no longer R114.2
- net LED_BLUE7: now also R103.2; no longer R132.2
- net LED_BLUE8: now also R117.2; no longer R150.2
- net LED_GREEN1: now also R17.2; no longer R19.2
- net LED_GREEN2: now also R36.2; no longer R45.2
- net LED_GREEN3: now also R50.2; no longer R63.2
- net LED_GREEN4: now also R64.2; no longer R81.2
- net LED_GREEN5: now also R78.2; no longer R99.2
- net LED_GREEN6: now also R92.2; no longer R117.2
- net LED_GREEN7: now also R106.2; no longer R135.2
- net LED_GREEN8: now also R120.2; no longer R153.2
- net LED_RED1: now also R10.2; no longer R17.2
- net LED_RED2: now also R34.2; no longer R43.2
- net LED_RED3: now also R48.2; no longer R61.2
- net LED_RED4: now also R62.2; no longer R79.2
- net LED_RED5: now also R76.2; no longer R97.2
- net LED_RED6: now also R90.2; no longer R115.2
- net LED_RED7: now also R104.2; no longer R133.2
- net LED_RED8: now also R118.2; no longer R151.2
- net LED_YELLOW1: now also R16.2; no longer R18.2
- net LED_YELLOW2: now also R35.2; no longer R44.2
- net LED_YELLOW3: now also R49.2; no longer R62.2
- net LED_YELLOW4: now also R63.2; no longer R80.2
- net LED_YELLOW5: now also R77.2; no longer R98.2
- net LED_YELLOW6: now also R91.2; no longer R116.2
- net LED_YELLOW7: now also R105.2; no longer R134.2
- net LED_YELLOW8: now also R119.2; no longer R152.2
- net N$1: now also R9.1; no longer R16.1
- net N$11: now also R33.1; no longer R42.1
- net N$12: now also R34.1; no longer R43.1
- net N$13: now also R35.1; no longer R44.1
- net N$14: now also R36.1; no longer R45.1
- net N$16: now also R47.1; no longer R60.1
- net N$17: now also R48.1; no longer R61.1
- net N$18: now also R49.1; no longer R62.1
- net N$19: now also R50.1; no longer R63.1
- net N$21: now also R61.1; no longer R78.1
- net N$22: now also R62.1; no longer R79.1
- net N$23: now also R63.1; no longer R80.1
- net N$24: now also R64.1; no longer R81.1
- net N$26: now also R75.1; no longer R96.1
- net N$27: now also R76.1; no longer R97.1
- net N$28: now also R77.1; no longer R98.1
- net N$29: now also R78.1; no longer R99.1
- net N$3: now also R10.1; no longer R17.1
- net N$31: now also R89.1; no longer R114.1
- net N$32: now also R90.1; no longer R115.1
- net N$33: now also R91.1; no longer R116.1
- net N$34: now also R92.1; no longer R117.1
- net N$36: now also R103.1; no longer R132.1
- net N$37: now also R104.1; no longer R133.1
- net N$38: now also R105.1; no longer R134.1
- net N$39: now also R106.1; no longer R135.1
- net N$4: now also R16.1; no longer R18.1
- net N$41: now also R117.1; no longer R150.1
- net N$42: now also R118.1; no longer R151.1
- net N$43: now also R119.1; no longer R152.1
- net N$44: now also R120.1; no longer R153.1
- net N$9: now also R17.1; no longer R19.1
- net QWIIC_SCL: no longer R24.1
- net QWIIC_SCL1: now also J10.4; no longer J11.4, R31.1
- net QWIIC_SCL2: now also J16.4; no longer J17.4, R49.1
- net QWIIC_SCL3: now also J22.4; no longer J23.4, R67.1
- net QWIIC_SCL4: now also J28.4; no longer J29.4, R85.1
- net QWIIC_SCL5: now also J34.4; no longer J35.4, R103.1
- net QWIIC_SCL6: now also J40.4; no longer J41.4, R121.1
- net QWIIC_SCL7: now also J46.4; no longer J47.4, R139.1
- net QWIIC_SCL8: now also J52.4; no longer J53.4, R157.1
- net QWIIC_SDA: no longer R23.1
- net QWIIC_SDA1: now also J10.3; no longer J11.3, R30.1
- net QWIIC_SDA2: now also J16.3; no longer J17.3, R48.1
- net QWIIC_SDA3: now also J22.3; no longer J23.3, R66.1
- net QWIIC_SDA4: now also J28.3; no longer J29.3, R84.1
- net QWIIC_SDA5: now also J34.3; no longer J35.3, R102.1
- net QWIIC_SDA6: now also J40.3; no longer J41.3, R120.1
- net QWIIC_SDA7: now also J46.3; no longer J47.3, R138.1
- net QWIIC_SDA8: now also J52.3; no longer J53.3, R156.1
- net SWDCK1: now also J11.4; no longer J12.4
- net SWDCK2: now also J17.4; no longer J18.4
- net SWDCK3: now also J23.4; no longer J24.4
- net SWDCK4: now also J29.4; no longer J30.4
- net SWDCK5: now also J35.4; no longer J36.4
- net SWDCK6: now also J41.4; no longer J42.4
- net SWDCK7: now also J47.4; no longer J48.4
- net SWDCK8: now also J53.4; no longer J54.4
- net SWDIO1: now also J11.2; no longer J12.2
- net SWDIO2: now also J17.2; no longer J18.2
- net SWDIO3: now also J23.2; no longer J24.2
- net SWDIO4: now also J29.2; no longer J30.2
- net SWDIO5: now also J35.2; no longer J36.2
- net SWDIO6: now also J41.2; no longer J42.2
- net SWDIO7: now also J47.2; no longer J48.2
- net SWDIO8: now also J53.2; no longer J54.2
- net UART-RX1: now also J6.3; no longer J7.3
- net UART-TX1: now also J6.2; no longer J7.2
- net VDD: now also J7.11, J7.4; no longer J6.11, J6.4, R10.2, R23.2, R24.2
- net VDD1: now also J10.2, J11.1, J12.11, J12.4, J8.1, R19.1, R20.1, R21.2; no longer J11.2, J12.1, J8.11, J8.4, J9.1, R30.2, R31.2, R32.1, R33.1, R34.2, R9.2
- net VDD2: now also J14.1, J16.2, J17.1, J18.11, J18.4, R24.2, R30.2, R31.2, R32.2, R38.1, R39.1; no longer J14.11, J14.4, J15.1, J17.2, J18.1, R37.2, R38.2, R39.2, R41.2, R48.2, R49.2, R50.1, R51.1, R52.2
- net VDD3: now also J20.1, J22.2, J23.1, J24.11, J24.4, R43.2, R44.2, R45.2, R46.2, R52.1, R53.1, R54.2; no longer J20.11, J20.4, J21.1, J23.2, J24.1, R55.2, R56.2, R57.2, R58.2, R59.2, R66.2, R67.2, R68.1, R69.1, R70.2
- net VDD4: now also J26.1, J28.2, J29.1, J30.11, J30.4, R57.2, R58.2, R59.2, R60.2, R66.1, R67.1, R68.2; no longer J26.11, J26.4, J27.1, J29.2, J30.1, R73.2, R74.2, R75.2, R76.2, R77.2, R84.2, R85.2, R86.1, R87.1, R88.2
- net VDD5: now also J32.1, J34.2, J35.1, J36.11, J36.4, R71.2, R72.2, R73.2, R74.2, R80.1, R81.1, R82.2; no longer J32.11, J32.4, J33.1, J35.2, J36.1, R102.2, R103.2, R104.1, R105.1, R106.2, R91.2, R92.2, R93.2, R94.2, R95.2
- net VDD6: now also J38.1, J40.2, J41.1, J42.11, J42.4, R85.2, R86.2, R87.2, R88.2, R94.1, R95.1, R96.2; no longer J38.11, J38.4, J39.1, J41.2, J42.1, R109.2, R110.2, R111.2, R112.2, R113.2, R120.2, R121.2, R122.1, R123.1, R124.2
- net VDD7: now also J44.1, J46.2, J47.1, J48.11, J48.4, R100.2, R101.2, R102.2, R108.1, R109.1, R110.2, R99.2; no longer J44.11, J44.4, J45.1, J47.2, J48.1, R127.2, R128.2, R129.2, R130.2, R131.2, R138.2, R139.2, R140.1, R141.1, R142.2
- net VDD8: now also J50.1, J52.2, J53.1, J54.11, J54.4, R113.2, R114.2, R115.2, R116.2, R122.1, R123.1, R124.2; no longer J50.11, J50.4, J51.1, J53.2, J54.1, R145.2, R146.2, R147.2, R148.2, R149.2, R156.2, R157.2, R158.1, R159.1, R160.2
- net ~1: now also J8.4; no longer J9.4
- net ~10: now also J32.5; no longer J33.5
- net ~11: now also J38.4; no longer J39.4
- net ~12: now also J38.5; no longer J39.5
- net ~13: now also J44.4; no longer J45.4
- net ~14: now also J44.5; no longer J45.5
- net ~15: now also J50.4; no longer J51.4
- net ~16: now also J50.5; no longer J51.5
- net ~2: now also J8.5; no longer J9.5
- net ~3: now also J14.4; no longer J15.4
- net ~4: now also J14.5; no longer J15.5
- net ~5: now also J20.4; no longer J21.4
- net ~6: now also J20.5; no longer J21.5
- net ~7: now also J26.4; no longer J27.4
- net ~8: now also J26.5; no longer J27.5
- net ~9: now also J32.4; no longer J33.4
- net ~A1: now also J8.3; no longer J9.3
- net ~A2: now also J14.3; no longer J15.3
- net ~A3: now also J20.3; no longer J21.3
- net ~A4: now also J26.3; no longer J27.3
- net ~A5: now also J32.3; no longer J33.3
- net ~A6: now also J38.3; no longer J39.3
- net ~A7: now also J44.3; no longer J45.3
- net ~A8: now also J50.3; no longer J51.3
- net ~AD33/SWO1: now also J11.6; no longer J12.6
- net ~AD33/SWO2: now also J17.6; no longer J18.6
- net ~AD33/SWO3: now also J23.6; no longer J24.6
- net ~AD33/SWO4: now also J29.6; no longer J30.6
- net ~AD33/SWO5: now also J35.6; no longer J36.6
- net ~AD33/SWO6: now also J41.6; no longer J42.6
- net ~AD33/SWO7: now also J47.6; no longer J48.6
- net ~AD33/SWO8: now also J53.6; no longer J54.6
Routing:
- net MIC_CLK5: track 91.7 -> 63.6 mm
- net MIC_CLK2: track 91.7 -> 63.6 mm
- net MIC_CLK4: track 91.7 -> 63.6 mm
- net MIC_CLK3: track 91.7 -> 63.6 mm
- net MIC_CLK1: track 91.7 -> 63.6 mm
- net MIC_CLK: track 91.7 -> 63.6 mm
- net MIC_CLK8: track 91.7 -> 63.6 mm
- net MIC_CLK7: track 91.7 -> 63.6 mm
- net MIC_CLK6: track 91.7 -> 63.6 mm
- net CAMERA_RESET: track 25.9 -> 0.00 mm
- net CAMERA_RESET8: track 25.9 -> 0.00 mm
- net CAMERA_RESET7: track 25.9 -> 0.00 mm
- net CAMERA_RESET6: track 25.9 -> 0.00 mm
- net CAMERA_RESET2: track 25.9 -> 0.00 mm
- net CAMERA_RESET1: track 25.9 -> 0.00 mm
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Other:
- board size 175.6 x 134.7 mm -> 177.7 x 134.7 mm
- board text added: "v21"
- board text removed: "v20"
